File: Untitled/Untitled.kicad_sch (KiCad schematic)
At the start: 3 parts

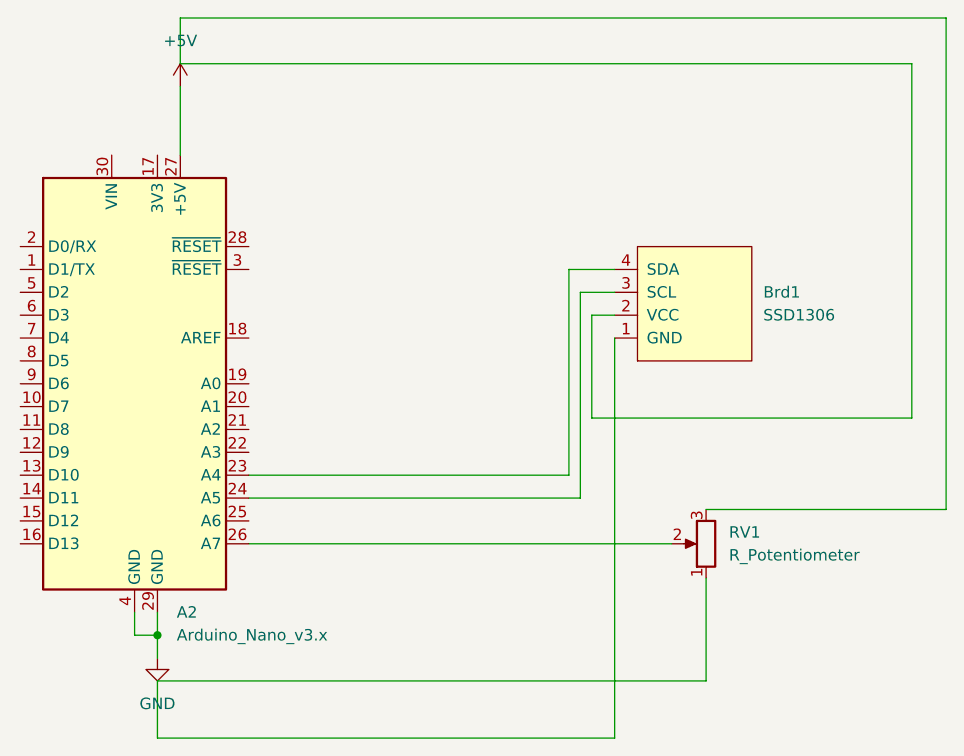
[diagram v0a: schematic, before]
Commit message: Added KiCad for the PCB
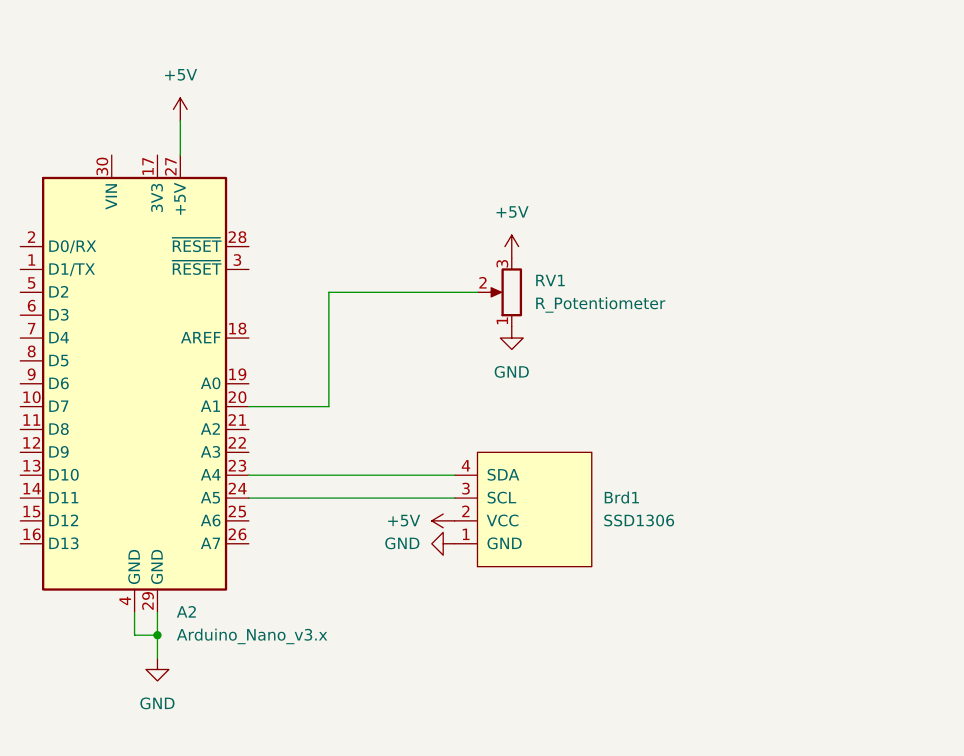
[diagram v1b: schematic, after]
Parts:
- A2: footprint Module:Arduino_Nano -> Module:Arduino_Nano_WithMountingHoles
- Brd1: footprint (none) -> Custom:Through-Hole Pads for SSD1306 0.96 Inch OLED Screen
- RV1: footprint (none) -> Custom:Through-Hole Pads 2.54mm
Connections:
- net +5V: now also Brd1.2 (VCC), RV1.3
- net GND: now also Brd1.1 (GND), RV1.1
- net at A2.20 (A1): now also RV1.2
- net at A2.26 (A7): no longer RV1.2
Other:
- moved on the sheet: Brd1, RV1
